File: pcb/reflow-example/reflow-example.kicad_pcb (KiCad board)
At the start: 2 copper layers, 47 x 43.8 mm, 50 parts, among them IC1 74LS393, IC2 NE555D, IC3 CD4511BNSR

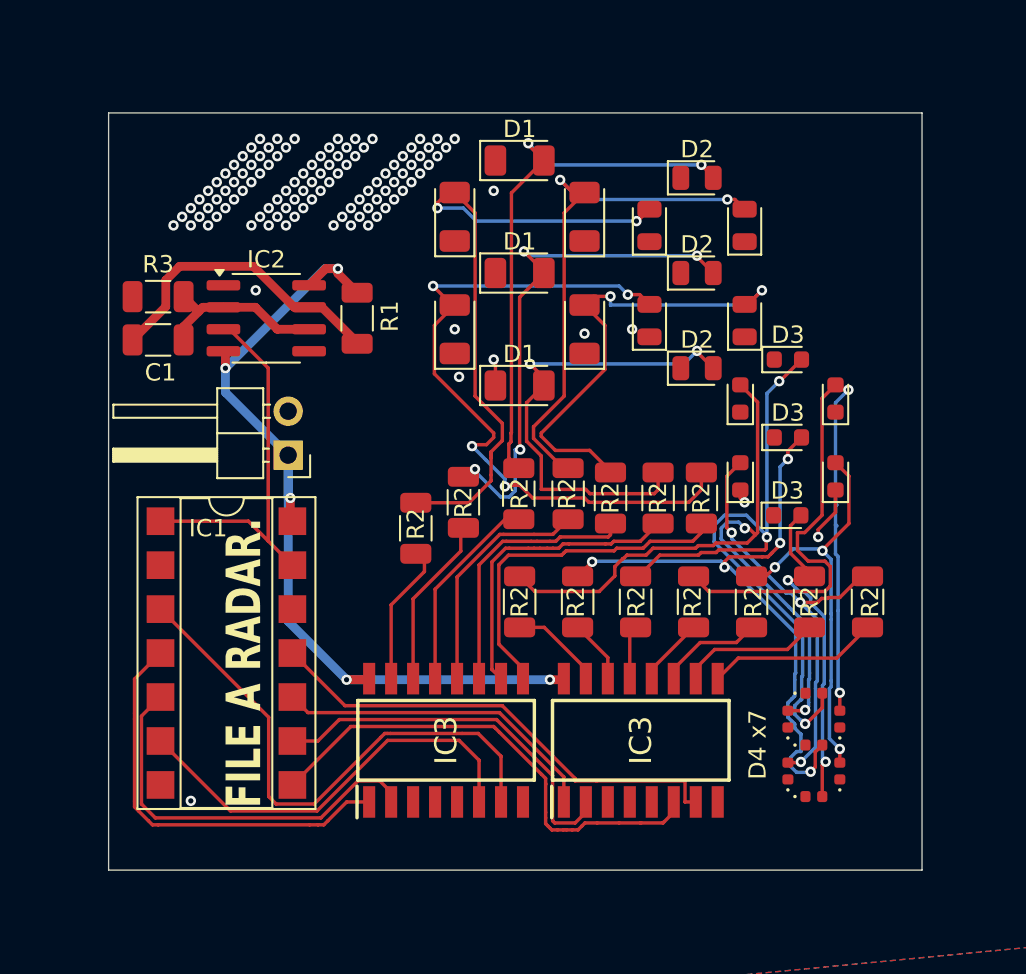
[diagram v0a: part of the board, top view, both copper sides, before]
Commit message: update:
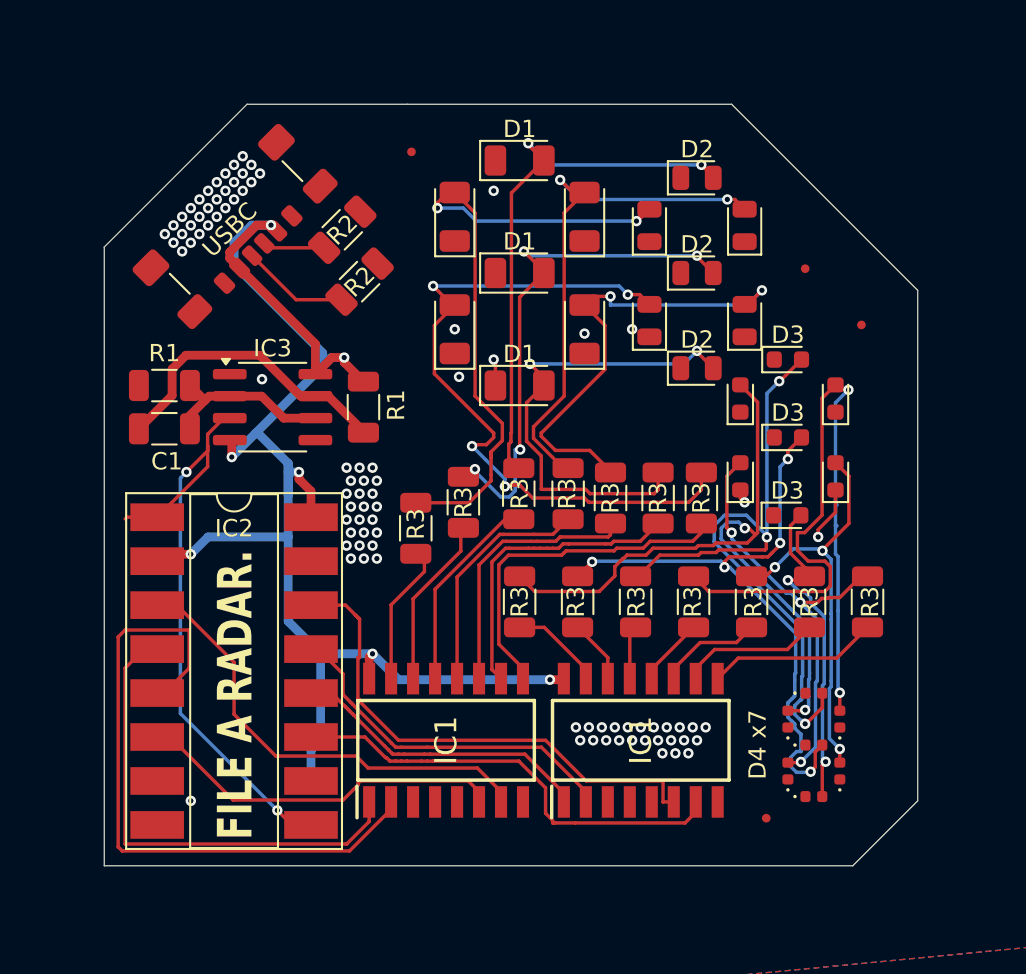
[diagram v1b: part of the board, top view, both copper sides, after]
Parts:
- removed the IC1 at (121.8, 100.0)
- removed V1: 5, Connector_PinHeader_2.54mm:PinHeader_1x02_P2.54mm_Horizontal
- added IC2: 4518, Package_DIP:DIP-16_W8.89mm_SMDSocket_LongPads, F.Cu at (122.2, 101.0)
- added R2: 5k1, Capacitor_SMD:C_1206_3216Metric, F.Cu at (129.5, 78.5)
- added R2: 5k1, Capacitor_SMD:C_1206_3216Metric, F.Cu at (128.5, 75.5)
- added REF**: Fiducial_0.5mm_Mask1.5mm, Fiducial:Fiducial_0.5mm_Mask1.5mm, F.Cu at (132.5, 71.0)
- added REF**: Fiducial_0.5mm_Mask1.5mm, Fiducial:Fiducial_0.5mm_Mask1.5mm, F.Cu at (155.2, 77.8)
- added REF**: Fiducial_0.5mm_Mask1.5mm, Fiducial:Fiducial_0.5mm_Mask1.5mm, F.Cu at (153.0, 109.5)
- added REF**: Fiducial_0.5mm_Mask1.5mm, Fiducial:Fiducial_0.5mm_Mask1.5mm, F.Cu at (158.5, 81.0)
- added USBC: USB_C_Receptacle_PowerOnly_6P, Connector_USB:USB_C_Receptacle_GCT_USB4135-GF-A_6P_TopMnt_Horizontal, F.Cu at (121.5, 74.5)
- D12: renamed from D3 x2
- moved C1 5.15 mm to (118.2, 84.5)
- moved IC3 5.15 mm to (124.5, 85.8)
- moved R1 5.15 mm to (118.2, 87.0)
- moved R1 5.15 mm to (129.7, 85.8)
- renumbered D3 to D10, D2 to D17, D1 to D18, D2 to D19, D1 to D20, D2 to D23, D1 to D24, D2 to D25, D1 to D26, D3 to D4, D3 to D6, IC3 to IC1, IC2 to IC3, R3 to R1, R2 to R3
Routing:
- net +5V: track 52.5 -> 90.0 mm, vias 5 -> 7
- net Net-(IC1-C_1): track 23.1 -> 38.3 mm
- net Net-(U1-Q): track 22.2 -> 35.9 mm, vias 0 -> 2
- net Net-(J1-CC2): track 0.00 -> 6.22 mm
- net Net-(IC1-A_1): track 31.9 -> 26.7 mm
- net Net-(IC1-B_1): track 24.0 -> 28.2 mm
- net Net-(J1-CC1): track 0.00 -> 3.56 mm
- net Net-(IC1-D_1): track 24.7 -> 21.5 mm
- net Net-(IC2-D_1): track 28.5 -> 30.2 mm
- net Net-(IC2-A_1): track 27.7 -> 26.1 mm
- net Net-(IC2-B_1): track 19.0 -> 17.5 mm
- net Net-(IC2-C_1): track 22.3 -> 21.1 mm
- net GND: vias 109 -> 88
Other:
- board size 47 x 43.8 mm -> 47 x 44 mm
